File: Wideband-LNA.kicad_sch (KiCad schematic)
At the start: 28 parts, among them J1 RF-IN, J2 RF-OUT, J3 USB_C_Receptacle_USB2.0_16P, U1 TQP3M9036, U2 AP2127K-ADJ

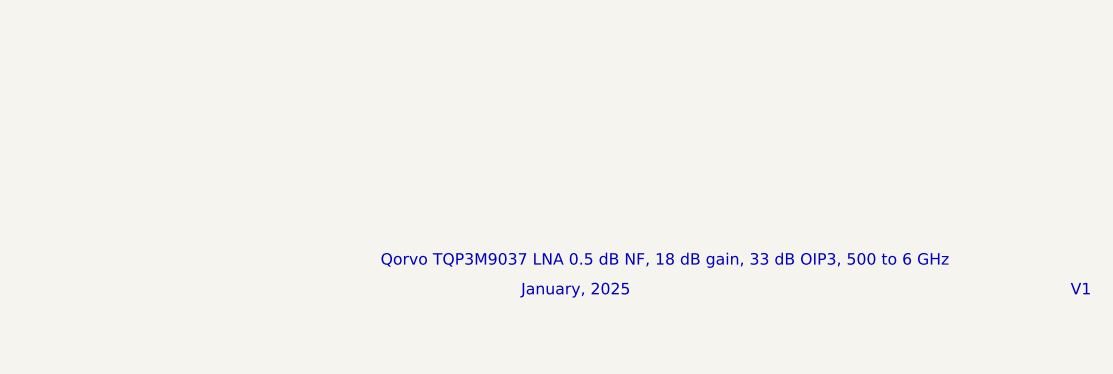
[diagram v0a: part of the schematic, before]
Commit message: Updated sheet titles to show Version and Git Branch
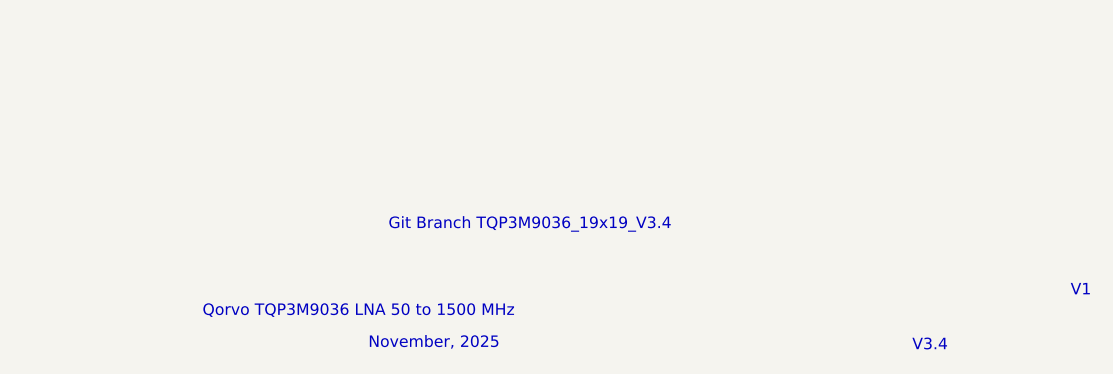
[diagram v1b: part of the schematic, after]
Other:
- note added: "Git Branch TQP3M9036_19x19_V3.4"
- note added: "November, 2025"
- note added: "Qorvo TQP3M9036 LNA 50 to 1500 MHz"
- note added: "V3.4"
- note removed: "January, 2025"
- note removed: "Qorvo TQP3M9037 LNA 0.5 dB NF, 18 dB gain, 33 dB OIP3, 500 to 6 GHz"
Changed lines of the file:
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@@
 	(generator_version "9.0")
 	(paper "USLetter")
+	(text "Git Branch TQP3M9036_19x19_V3.4"
+		(exclude_from_sim no)
+		(at 209.042 185.928 0)
+		(effects
+			(font
+				(size 1.27 1.27)
+			)
+		)
+	)
 	(text "V1\n"
 		(exclude_from_sim no)
@@
 		)
 	)
-	(text "January, 2025"
+	(text "November, 2025"
 		(exclude_from_sim no)
-		(at 214.122 193.294 0)
+		(at 198.374 199.136 0)
+		(effects
+			(font
+				(size 1.27 1.27)
+			)
+		)
+	)
+	(text "V3.4"
+		(exclude_from_sim no)
+		(at 253.492 199.39 0)
 		(effects
 			(font
@@
 		)
 	)
-	(text "Qorvo TQP3M9037 LNA 0.5 dB NF, 18 dB gain, 33 dB OIP3, 500 to 6 GHz"
+	(text "Qorvo TQP3M9036 LNA 50 to 1500 MHz"
 		(exclude_from_sim no)
-		(at 224.028 189.992 0)
+		(at 189.992 195.58 0)
 		(effects
 			(font
